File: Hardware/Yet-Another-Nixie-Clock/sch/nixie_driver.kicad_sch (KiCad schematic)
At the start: 22 parts, among them Q10 BF820, Q11 BF820, Q12 BF820, Q13 BF820, Q4 BF820, Q5 BF820, Q6 BF820, Q7 BF820, Q8 BF820, Q9 BF820, U15 74HC237, U17 74HC237

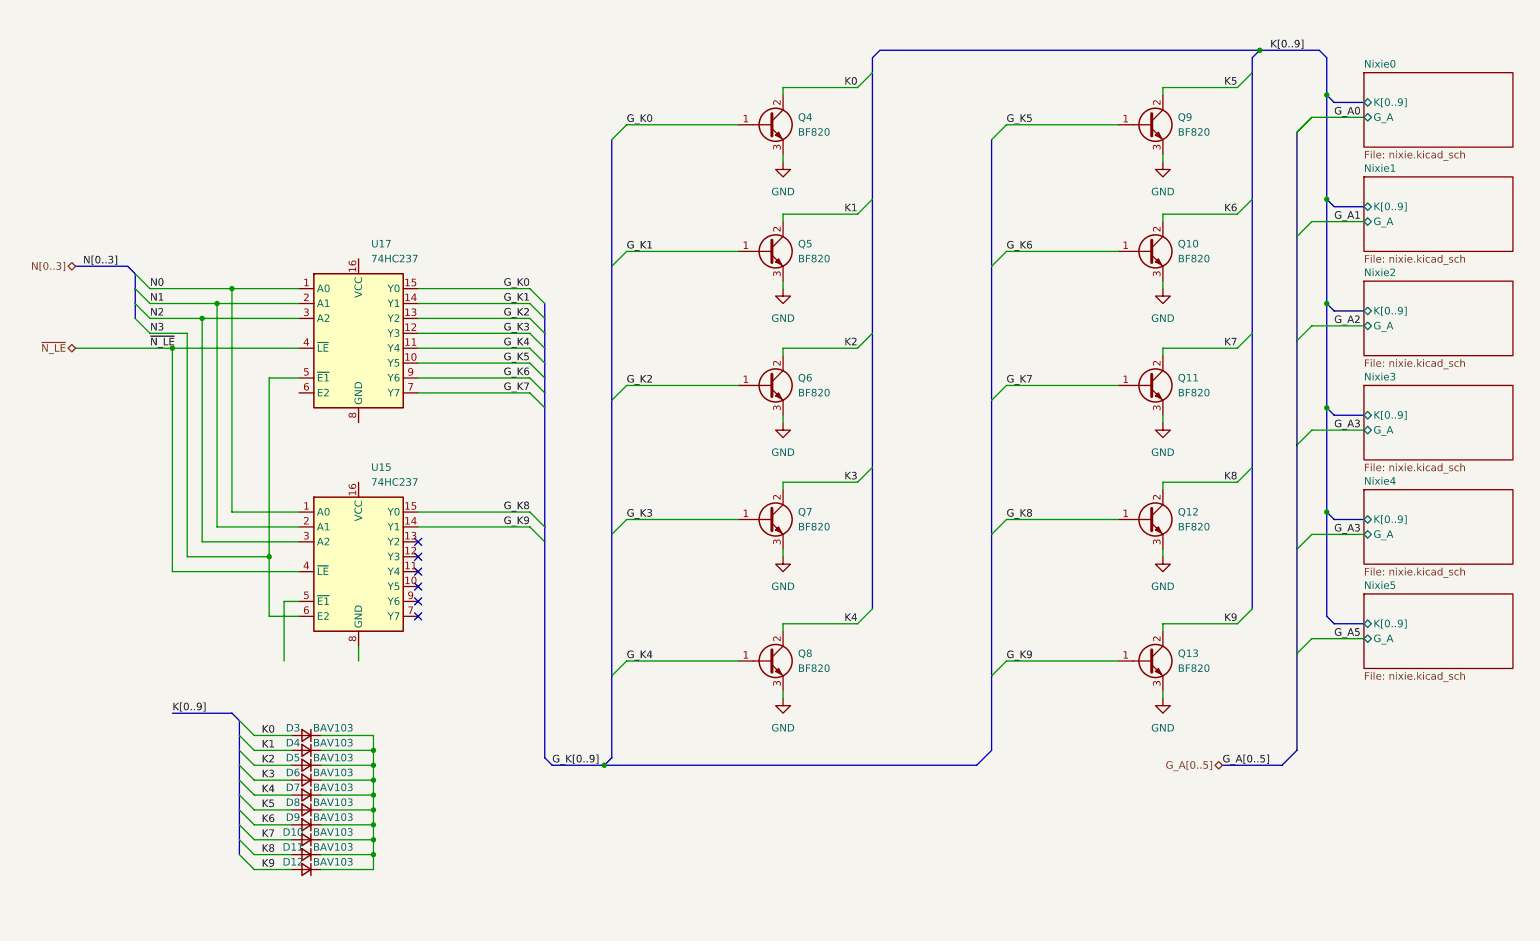
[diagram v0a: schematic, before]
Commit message: Schematic work
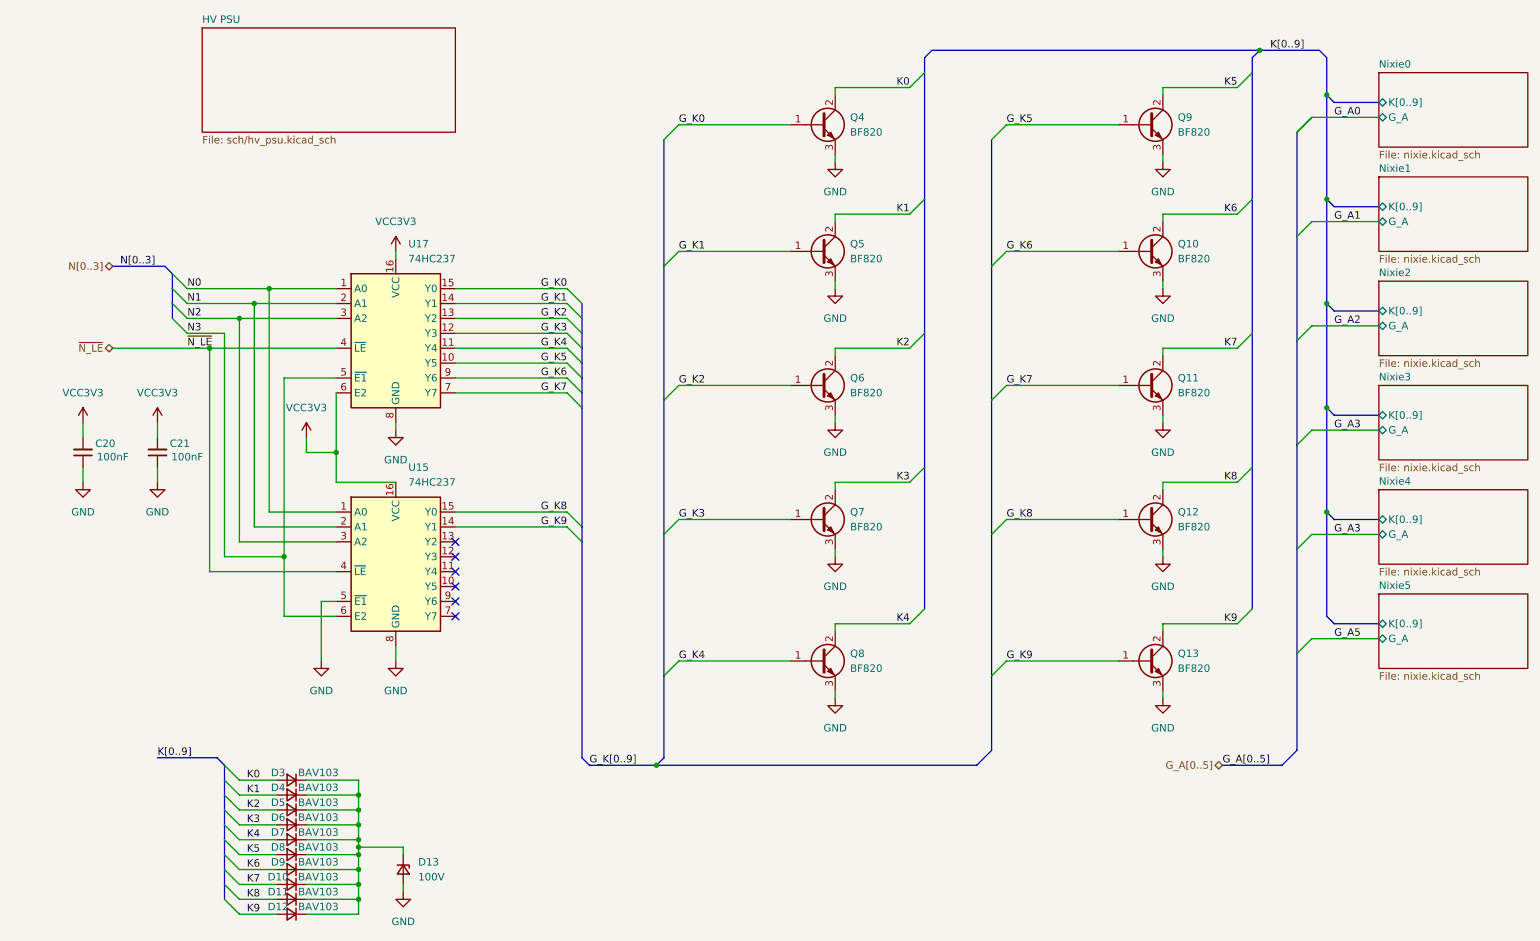
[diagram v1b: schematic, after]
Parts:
- added C20, C21: 100nF, Capacitor_SMD:C_0603_1608Metric, symbol Device:C_Small
- added D13: 100V, Diode_SMD:D_SMA, symbol Device:D_Zener_Small
- U15, U17: LCSC (none) -> C2674656
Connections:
- net GND: now also U15.5 (~{E1}), U15.8 (GND), U17.8 (GND), C20.1, C21.1, D13.2 (A)
- net at D10.1 (K), D11.1 (K), D12.1 (K)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: now also D13.1 (K)
- net VCC3V3: now reaches U17.16 (VCC)
- net VCC3V3: now also U15.16 (VCC), U17.6 (E2), C20.2, C21.2
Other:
- added sheet HV PSU (sch/hv_psu.kicad_sch)
- moved on the sheet: D10, D11, D12, D3, D4, D5, D6, D7, D8, D9, Q4, Q5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
